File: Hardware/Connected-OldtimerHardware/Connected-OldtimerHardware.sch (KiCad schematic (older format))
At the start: 20 parts, among them J1 CAN_Bus_Connector, J2 MainConnector, J3 NextionConnector, Q1 2N3906, U1 ParticleElectron, U2 TSR_2-2450, U3 CANTranceiverModule, U4 AdafruitFRAM, U5 AdafruitUltimateGPS, U6 MotionSensor, U7 SFH618A-2

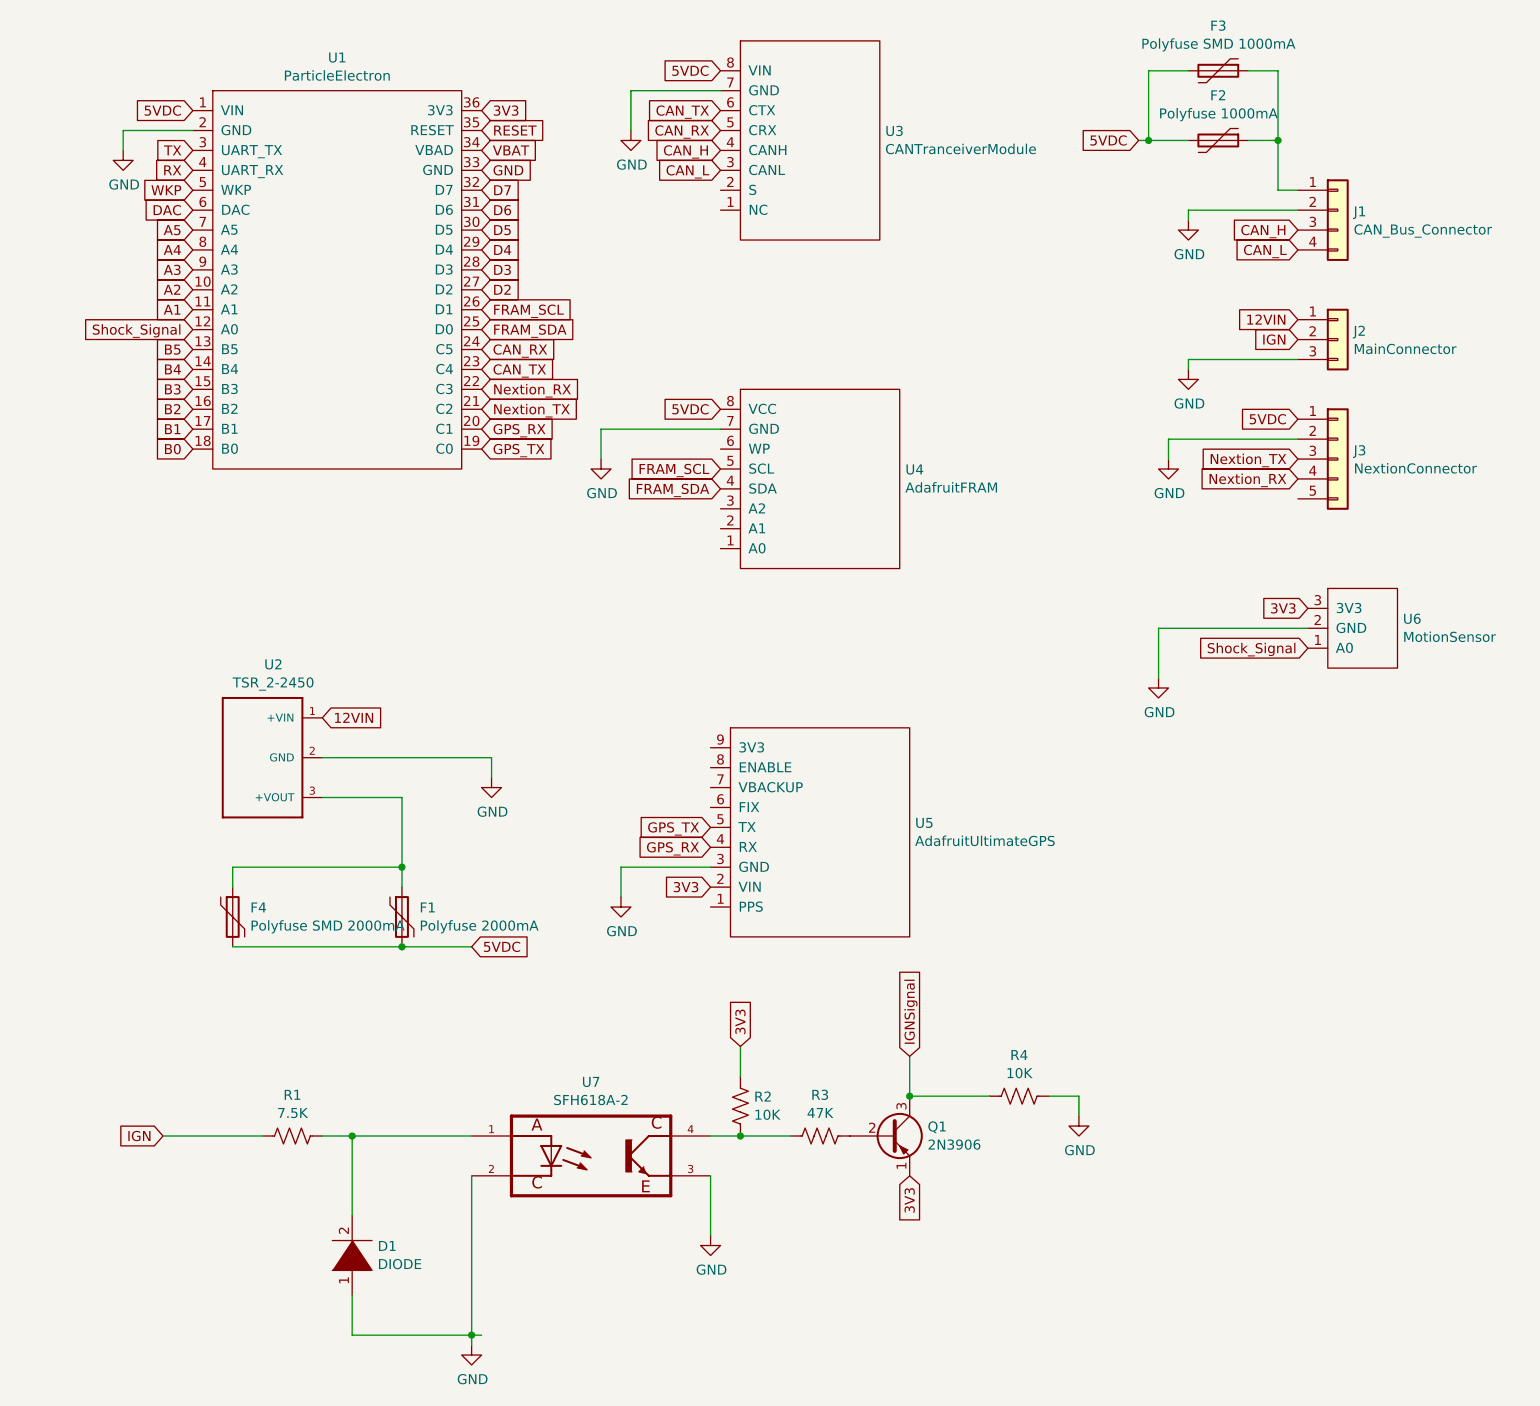
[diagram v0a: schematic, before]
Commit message: layout v1
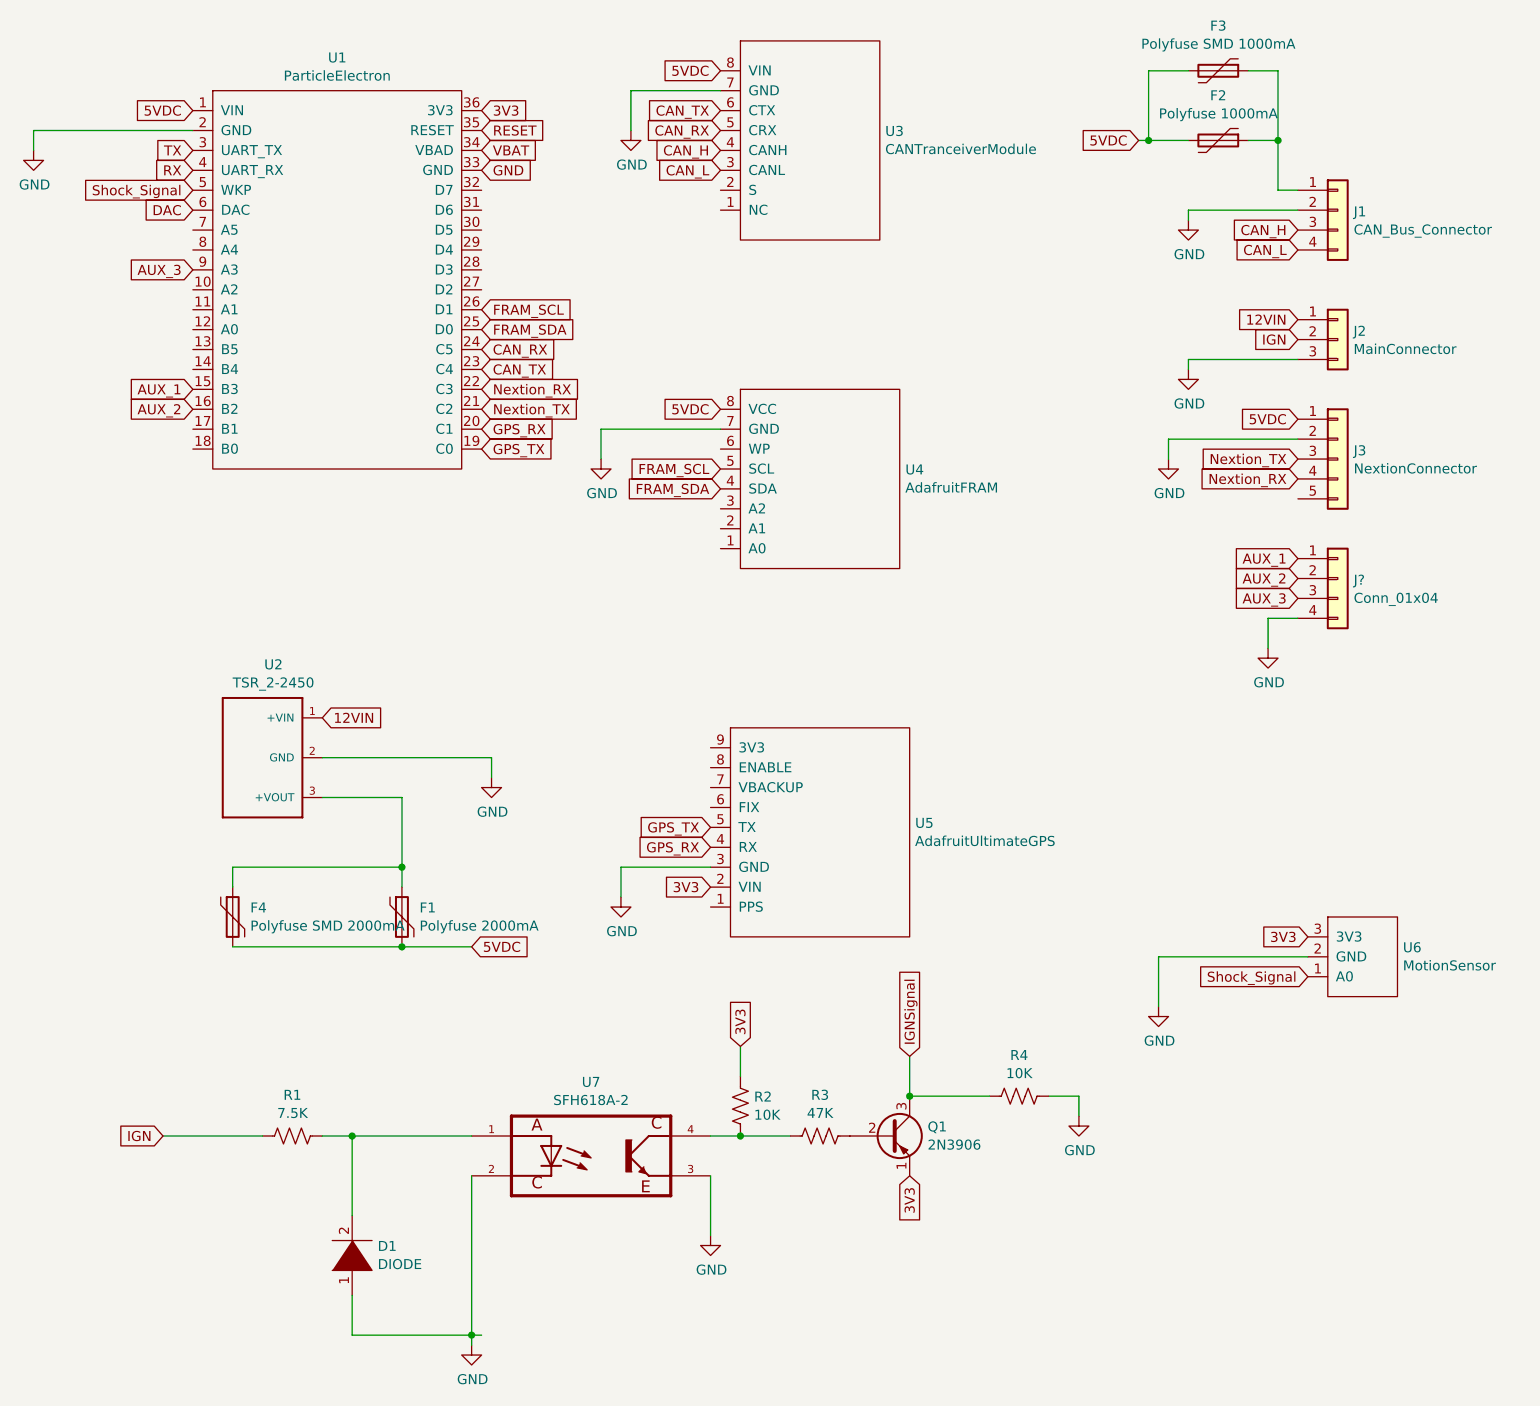
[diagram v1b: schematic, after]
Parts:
- added J?: Conn_01x04, symbol Connector_Generic:Conn_01x04
- F4: footprint Fuse:Fuse_Littelfuse-LVR200 -> Capacitor_SMD:C_1210_3225Metric_Pad1.42x2.65mm_HandSolder
- J1: footprint Connector_JST:JST_EH_B04B-EH-A_1x04_P2.50mm_Vertical -> Connector_JST:JST_XH_B04B-XH-A_1x04_P2.50mm_Vertical
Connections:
- net WKP is gone; now on net Shock_Signal: U1.5 (WKP)
- net GND: now also J?.4 (Pin_4)
- net Shock_Signal: no longer U1.12 (A0)
- net A1: no longer names the net of U1.11 (A1)
- net A2: no longer names the net of U1.10 (A2)
- net A3 renamed AUX_3
- net AUX_3: now also J?.3 (Pin_3)
- net A4: no longer names the net of U1.8 (A4)
- net A5: no longer names the net of U1.7 (A5)
- net B0: no longer names the net of U1.18 (B0)
- net B1: no longer names the net of U1.17 (B1)
- net B2 renamed AUX_2
- net AUX_2: now also J?.2 (Pin_2)
- net B3 renamed AUX_1
- net AUX_1: now also J?.1 (Pin_1)
- net B4: no longer names the net of U1.14 (B4)
- net B5: no longer names the net of U1.13 (B5)
- net D2: no longer names the net of U1.27 (D2)
- net D3: no longer names the net of U1.28 (D3)
- net D4: no longer names the net of U1.29 (D4)
- net D5: no longer names the net of U1.30 (D5)
- net D6: no longer names the net of U1.31 (D6)
- net D7: no longer names the net of U1.32 (D7)
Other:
- moved on the sheet: U6
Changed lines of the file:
@@
 Text GLabel 1500 1350 0    50   Input ~ 0
 RX
-Text GLabel 1500 1450 0    50   Input ~ 0
-WKP
 Text GLabel 1500 1550 0    50   Input ~ 0
 DAC
-Text GLabel 1500 1650 0    50   Input ~ 0
-A5
-Text GLabel 1500 1750 0    50   Input ~ 0
-A4
-Text GLabel 1500 1850 0    50   Input ~ 0
-A3
-Text GLabel 1500 1950 0    50   Input ~ 0
-A2
-Text GLabel 1500 2050 0    50   Input ~ 0
-A1
-Text GLabel 1500 2150 0    50   Input ~ 0
+Text GLabel 1500 1450 0    50   Input ~ 0
 Shock_Signal
-Text GLabel 1500 2250 0    50   Input ~ 0
-B5
-Text GLabel 1500 2350 0    50   Input ~ 0
-B4
-Text GLabel 1500 2450 0    50   Input ~ 0
-B3
-Text GLabel 1500 2550 0    50   Input ~ 0
-B2
-Text GLabel 1500 2650 0    50   Input ~ 0
-B1
-Text GLabel 1500 2750 0    50   Input ~ 0
-B0
 Text GLabel 4150 2550 0    50   Input ~ 0
 5VDC
@@
 F 0 "J1" H 7330 1542 50  0000 L CNN
 F 1 "CAN_Bus_Connector" H 7330 1451 50  0000 L CNN
-F 2 "Connector_JST:JST_EH_B04B-EH-A_1x04_P2.50mm_Vertical" H 7250 1550 50  0001 C CNN
+F 2 "Connector_JST:JST_XH_B04B-XH-A_1x04_P2.50mm_Vertical" H 7250 1550 50  0001 C CNN
 F 3 "~" H 7250 1550 50  0001 C CNN
 	1    7250 1550
@@
 Text GLabel 7050 1750 0    50   Input ~ 0
 CAN_L
-Text GLabel 7100 3550 0    50   Input ~ 0
+Text GLabel 7100 5200 0    50   Input ~ 0
 3V3
-Text GLabel 7100 3750 0    50   Input ~ 0
+Text GLabel 7100 5400 0    50   Input ~ 0
 Shock_Signal
 $Comp
@@
 Text GLabel 2950 1350 2    50   Input ~ 0
 GND
-Text GLabel 2950 1450 2    50   Input ~ 0
-D7
-Text GLabel 2950 1550 2    50   Input ~ 0
-D6
-Text GLabel 2950 1650 2    50   Input ~ 0
-D5
-Text GLabel 2950 1750 2    50   Input ~ 0
-D4
-Text GLabel 2950 1850 2    50   Input ~ 0
-D3
-Text GLabel 2950 1950 2    50   Input ~ 0
-D2
 Text GLabel 2950 2050 2    50   Input ~ 0
 FRAM_SCL
@@
 L Connected-OldtimerHardware-rescue:MotionSensor-HeathsComponents U6
 U 1 1 5D6D1163
-P 7500 3650
-F 0 "U6" H 7577 3696 50  0000 L CNN
-F 1 "MotionSensor" H 7577 3605 50  0000 L CNN
-F 2 "heathsfootprints:ShockSensor" H 7500 3650 50  0001 C CNN
-F 3 "" H 7500 3650 50  0001 C CNN
-	1    7500 3650
+P 7500 5300
+F 0 "U6" H 7577 5346 50  0000 L CNN
+F 1 "MotionSensor" H 7577 5255 50  0000 L CNN
+F 2 "heathsfootprints:ShockSensor" H 7500 5300 50  0001 C CNN
+F 3 "" H 7500 5300 50  0001 C CNN
+	1    7500 5300
 	1    0    0    -1
 $EndComp
@@
 L power:GND #PWR0109
 U 1 1 5D6E51A5
-P 6350 3900
-F 0 "#PWR0109" H 6350 3650 50  0001 C CNN
-F 1 "GND" H 6355 3727 50  0000 C CNN
-F 2 "" H 6350 3900 50  0001 C CNN
-F 3 "" H 6350 3900 50  0001 C CNN
-	1    6350 3900
-	1    0    0    -1
-$EndComp
-Wire Wire Line
-	6350 3650 6350 3900
+P 6350 5550
+F 0 "#PWR0109" H 6350 5300 50  0001 C CNN
+F 1 "GND" H 6355 5377 50  0000 C CNN
+F 2 "" H 6350 5550 50  0001 C CNN
+F 3 "" H 6350 5550 50  0001 C CNN
+	1    6350 5550
+	1    0    0    -1
+$EndComp
+Wire Wire Line
+	6350 5300 6350 5550
 Wire Wire Line
 	7050 2700 6400 2700
@@
 L power:GND #PWR0112
 U 1 1 5D6E6E4F
-P 1150 1250
-F 0 "#PWR0112" H 1150 1000 50  0001 C CNN
-F 1 "GND" H 1155 1077 50  0000 C CNN
-F 2 "" H 1150 1250 50  0001 C CNN
-F 3 "" H 1150 1250 50  0001 C CNN
-	1    1150 1250
-	1    0    0    -1
-$EndComp
-Wire Wire Line
-	1500 1150 1150 1150
-Wire Wire Line
-	1150 1150 1150 1250
+P 700 1250
+F 0 "#PWR0112" H 700 1000 50  0001 C CNN
+F 1 "GND" H 705 1077 50  0000 C CNN
+F 2 "" H 700 1250 50  0001 C CNN
+F 3 "" H 700 1250 50  0001 C CNN
+	1    700  1250
+	1    0    0    -1
+$EndComp
+Wire Wire Line
+	700  1150 700  1250
 $Comp
 L Device:Polyfuse F2
@@
 	2900 5250 2550 5250
 Wire Wire Line
-	6350 3650 7100 3650
+	6350 5300 7100 5300
 Wire Wire Line
 	3550 2650 4150 2650
@@
 F 0 "F4" H 1788 5146 50  0000 L CNN
 F 1 "Polyfuse SMD 2000mA" H 1788 5055 50  0000 L CNN
-F 2 "Fuse:Fuse_Littelfuse-LVR200" H 1750 4900 50  0001 L CNN
+F 2 "Capacitor_SMD:C_1210_3225Metric_Pad1.42x2.65mm_HandSolder" H 1750 4900 50  0001 L CNN
 F 3 "~" H 1700 5100 50  0001 C CNN
 	1    1700 5100
@@
 	2550 5250 1700 5250
 Connection ~ 2550 5250
+$Comp
+L power:GND #PWR?
+U 1 1 5D70C303
+P 6900 3750
+F 0 "#PWR?" H 6900 3500 50  0001 C CNN
+F 1 "GND" H 6905 3577 50  0000 C CNN
+F 2 "" H 6900 3750 50  0001 C CNN
+F 3 "" H 6900 3750 50  0001 C CNN
+	1    6900 3750
+	1    0    0    -1
+$EndComp
+Wire Wire Line
+	6900 3750 6900 3600
+Wire Wire Line
+	6900 3600 7050 3600
+Text GLabel 7050 3300 0    50   Input ~ 0
+AUX_1
+Text GLabel 7050 3400 0    50   Input ~ 0
+AUX_2
+Text GLabel 7050 3500 0    50   Input ~ 0
+AUX_3
+Text GLabel 1500 2450 0    50   Input ~ 0
+AUX_1
+Text GLabel 1500 2550 0    50   Input ~ 0
+AUX_2
+Wire Wire Line
+	700  1150 1500 1150
+Text GLabel 1500 1850 0    50   Input ~ 0
+AUX_3
+$Comp
+L Connector_Generic:Conn_01x04 J?
+U 1 1 5D717741
+P 7250 3400
+F 0 "J?" H 7330 3392 50  0000 L CNN
+F 1 "Conn_01x04" H 7330 3301 50  0000 L CNN
+F 2 "" H 7250 3400 50  0001 C CNN
+F 3 "~" H 7250 3400 50  0001 C CNN
+	1    7250 3400
+	1    0    0    -1
+$EndComp
 $EndSCHEMATC
